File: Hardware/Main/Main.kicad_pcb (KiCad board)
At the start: 4 copper layers, 19 parts, among them J1 POWERBOARD, SW1 SW_Push, SW2 SW_Push, SW3 SW_Push, SW4 RotaryEncoder_Switch, SW5 SW_Push, U1 TFT_ST7789, U2 ESP32-WROOM-32D

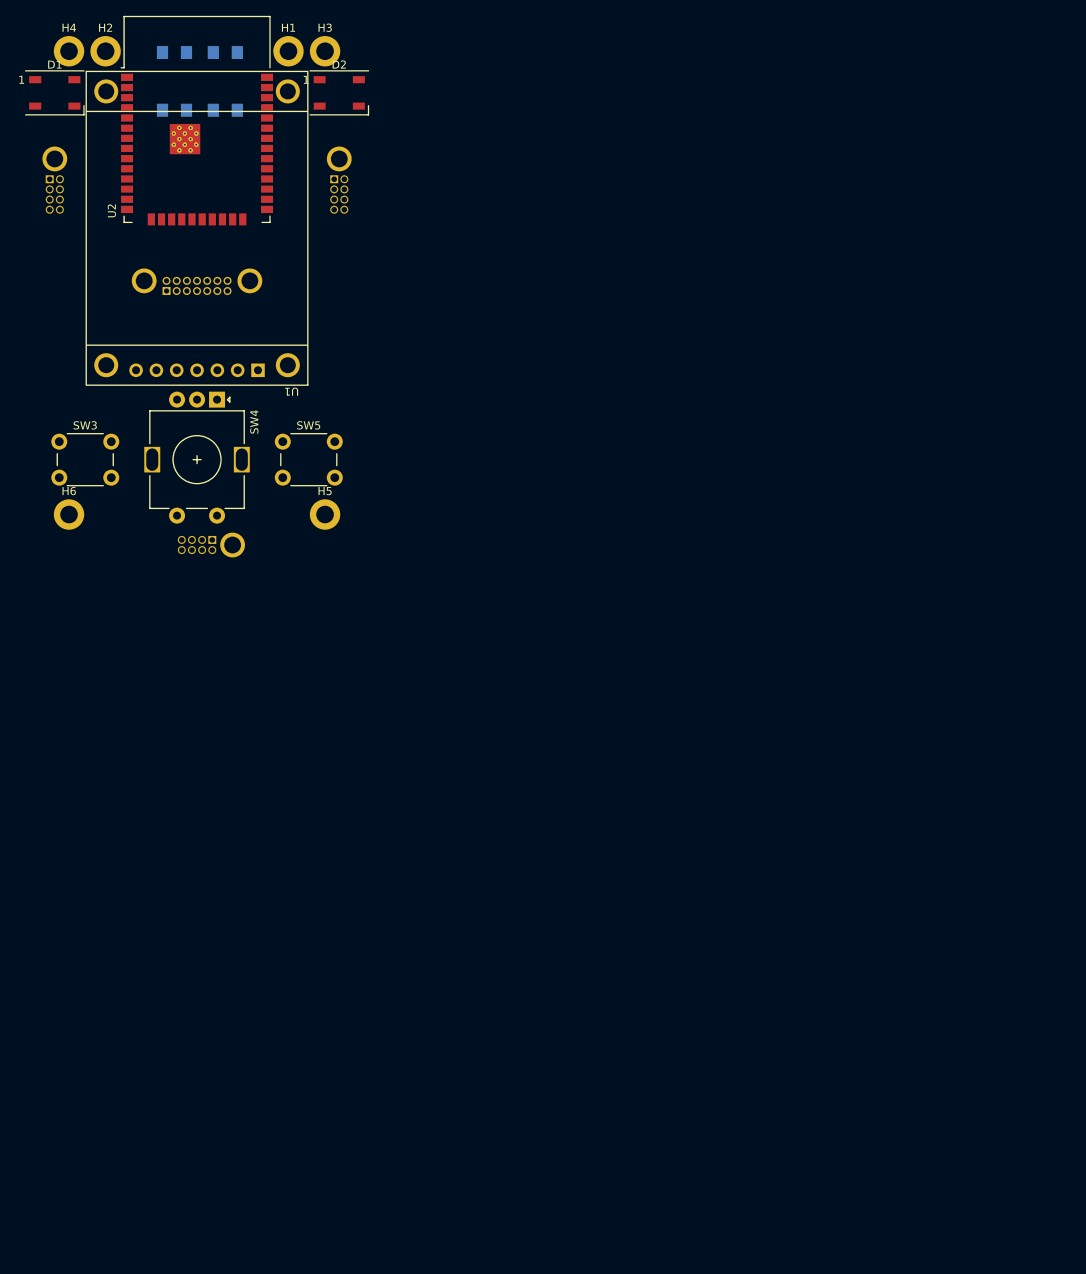
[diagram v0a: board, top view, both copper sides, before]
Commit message: Mainboard edge cuts
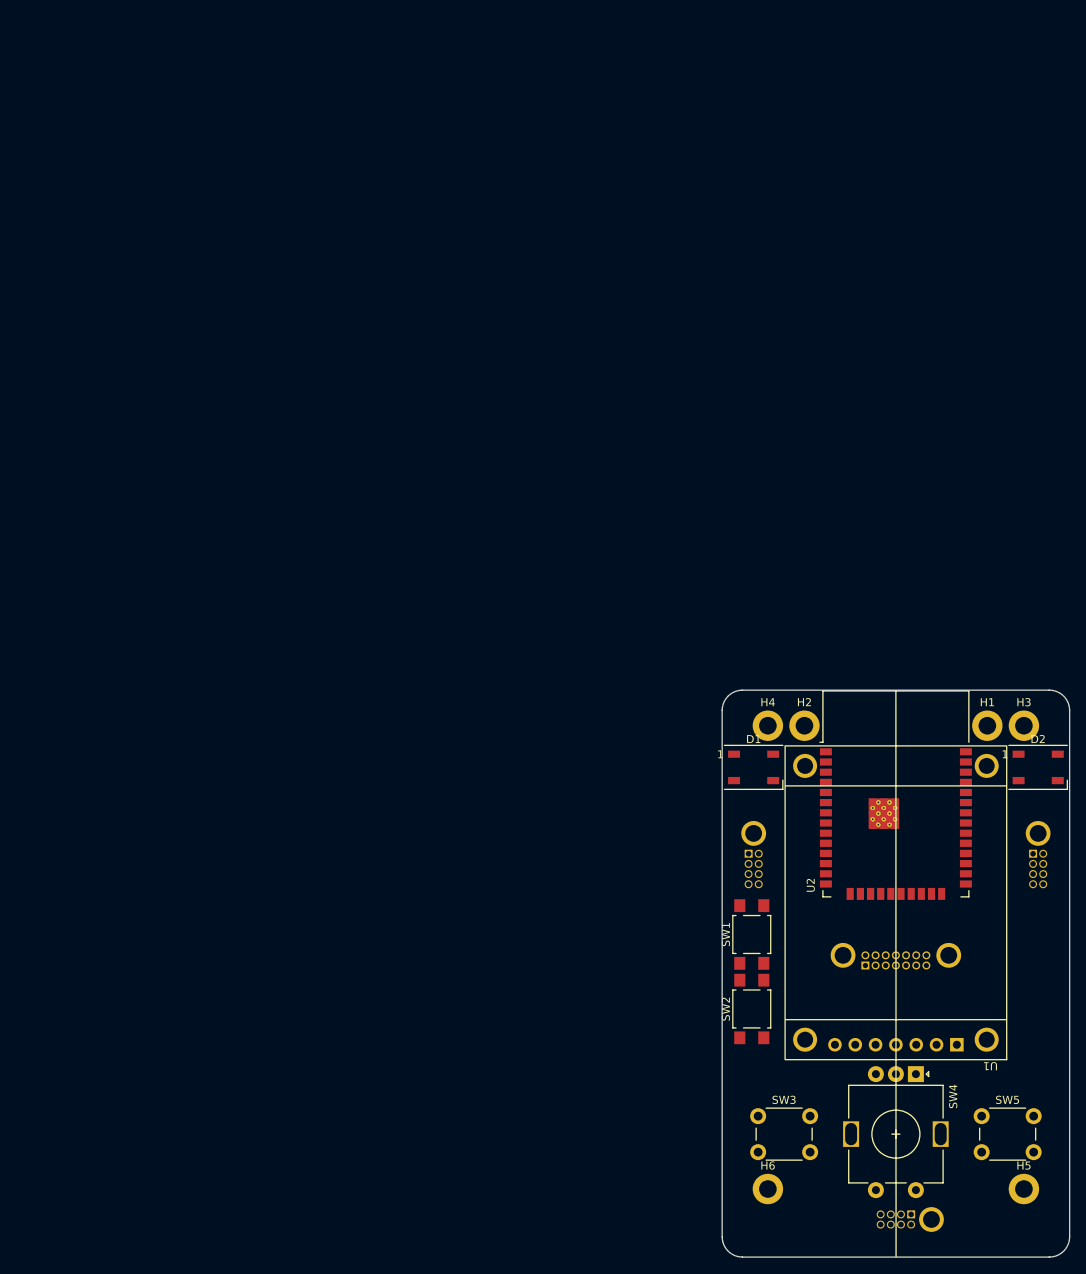
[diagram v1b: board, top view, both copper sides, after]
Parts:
- SW1, SW2: moved to F.Cu
- moved SW2 133.3 mm to (69.3, 91.0), turned to 90 degrees
- moved SW1 128.8 mm to (69.3, 81.7), turned to 90 degrees
- moved D1 121.4 mm to (69.6, 60.8)
- moved D2 121.4 mm to (105.1, 60.8)
- moved H1 121.4 mm to (98.8, 55.6)
- moved H2 121.4 mm to (75.9, 55.6)
- moved H3 121.4 mm to (103.4, 55.6)
- moved H4 121.4 mm to (71.4, 55.6)
- moved H5 121.4 mm to (103.4, 113.5)
- moved J1 121.4 mm to (87.4, 84.9)
- moved Per1 121.4 mm to (87.4, 117.3)
- moved Per2 121.4 mm to (105.1, 73.5)
- moved Per3 121.4 mm to (69.6, 73.5)
- moved SW3 121.4 mm to (70.1, 104.4)
- moved SW4 121.4 mm to (89.9, 99.2)
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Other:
- board outline added: 43.4 x 70.9 mm
